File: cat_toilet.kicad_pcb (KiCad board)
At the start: 2 copper layers, 38 x 35 mm, 30 parts, among them J1 Conn_01x02, J2 ISP, J3 GP2Y0A41SK0F, Q1 S8050, SW1 EN Btn, SW2 EN Btn, SW3 Pairing Btn, U1 NCP187, U2 USB_CType_6Pin, U3 MCP73831, U4 ESP32-WROOM-32E

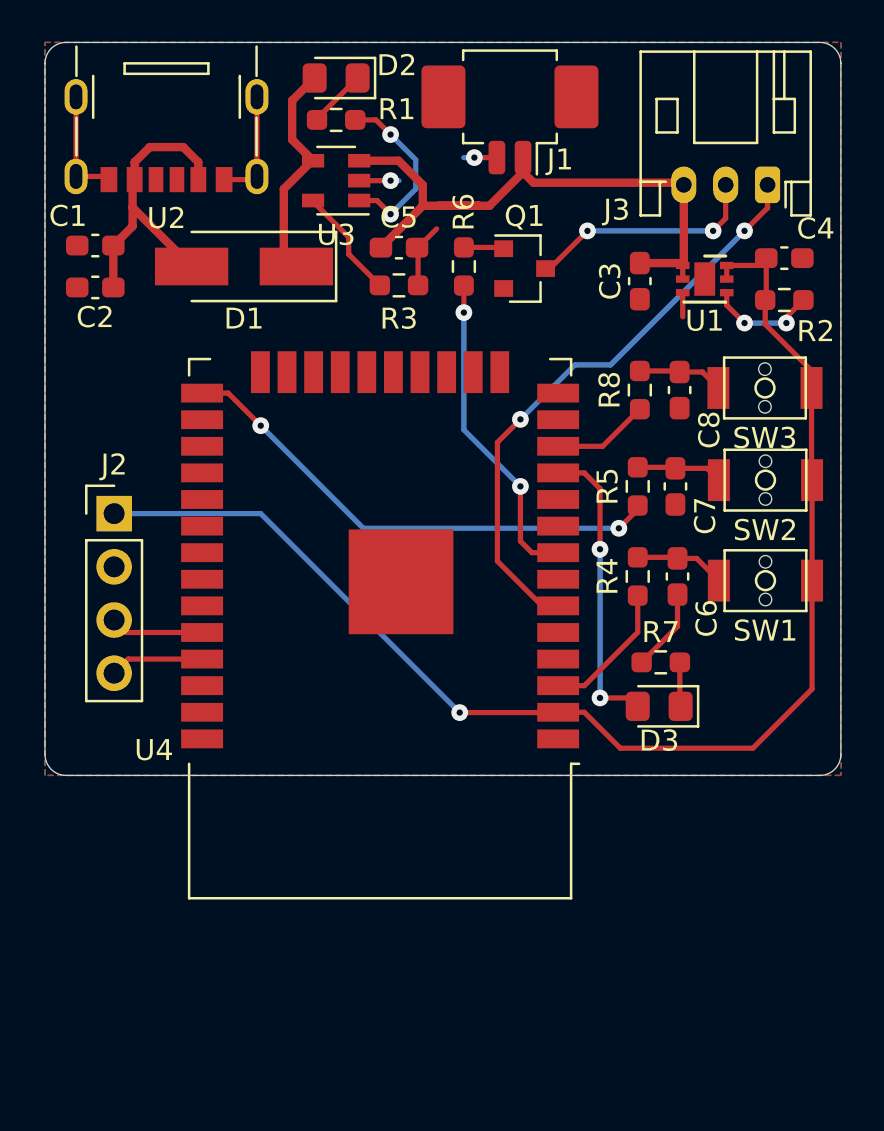
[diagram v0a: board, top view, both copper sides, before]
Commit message: 2021-12-14
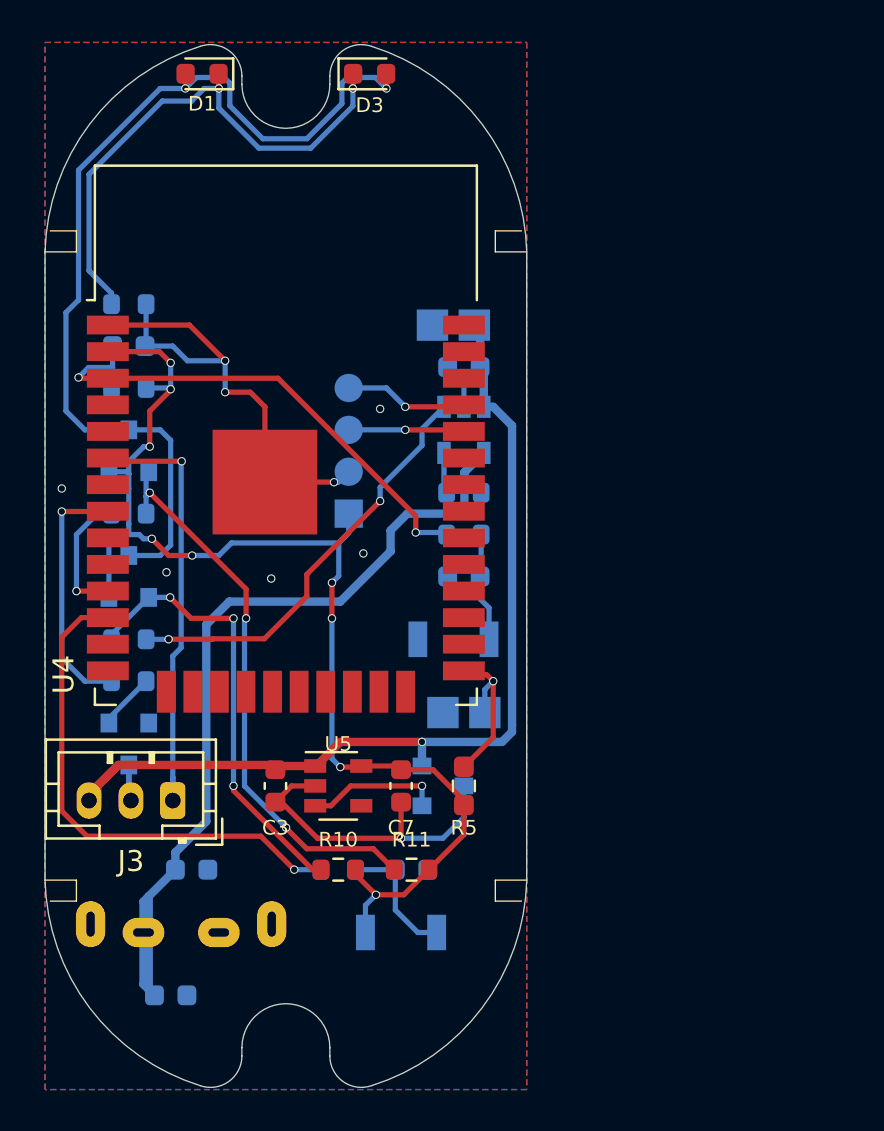
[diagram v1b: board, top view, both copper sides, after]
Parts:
- removed C4: 10u, Capacitor_SMD:C_0603_1608Metric_Pad1.08x0.95mm_HandSolder
- removed D2: LED/2012, LED_SMD:LED_0805_2012Metric_Pad1.15x1.40mm_HandSolder
- removed SW3: Pairing Btn, ali_Switch:NW3-A03-05
- added C9: 1u, Capacitor_SMD:C_0603_1608Metric, B.Cu at (4.00, 14.5)
- added Q2: BC856B,215, Package_TO_SOT_SMD:SOT-23, B.Cu at (4.00, 25.5)
- added Q3: BC856B,215, Package_TO_SOT_SMD:SOT-23, B.Cu at (4.00, 19.5)
- added R10: 33k, Resistor_SMD:R_0603_1608Metric, F.Cu at (14.0, 39.5)
- added R11: 33k, Resistor_SMD:R_0603_1608Metric, F.Cu at (17.5, 39.5)
- added R9: 33k, Resistor_SMD:R_0603_1608Metric, B.Cu at (4.00, 22.5)
- added TP1: TestPoint_2Pole, tp:boot, B.Cu at (19.0, 32.0)
- added U5: MCP1802T-3302I/OT, Package_TO_SOT_SMD:SOT-23-5, F.Cu at (14.0, 35.5)
- C1, C2, C5, C6, C8: footprint Capacitor_SMD:C_0603_1608Metric_Pad1.08x0.95mm_HandSolder -> Capacitor_SMD:C_0603_1608Metric; moved to B.Cu
- C3, C7: footprint Capacitor_SMD:C_0603_1608Metric_Pad1.08x0.95mm_HandSolder -> Capacitor_SMD:C_0603_1608Metric
- D1: value SK24/SMA -> LED/1608; footprint Diode_SMD:D_SMA_Handsoldering -> LED_SMD:LED_0603_1608Metric
- D3: value LED -> LED/1608; footprint LED_SMD:LED_0805_2012Metric_Pad1.15x1.40mm_HandSolder -> LED_SMD:LED_0603_1608Metric
- J1: value Conn_01x02 -> Batt; footprint Connector_Molex:Molex_PicoBlade_53261-0271_1x02-1MP_P1.25mm_Horizontal -> tp:boot; moved to B.Cu
- J2: footprint Connector_PinHeader_2.54mm:PinHeader_1x04_P2.54mm_Vertical -> Connector_PinHeader_2.00mm:PinHeader_1x04_P2.00mm_Vertical; moved to B.Cu
- J3: footprint Connector_JST:JST_PH_S3B-PH-K_1x03_P2.00mm_Horizontal -> Connector_JST:JST_PH_B3B-PH-K_1x03_P2.00mm_Vertical
- Q1: value S8050 -> npn; moved to B.Cu
- R1: value 510 -> 10k; footprint Resistor_SMD:R_0603_1608Metric_Pad0.98x0.95mm_HandSolder -> Resistor_SMD:R_0603_1608Metric; moved to B.Cu
- R2: value 100k -> 33k; footprint Resistor_SMD:R_0603_1608Metric_Pad0.98x0.95mm_HandSolder -> Resistor_SMD:R_0603_1608Metric; moved to B.Cu
- R3, R6, R7, R8: footprint Resistor_SMD:R_0603_1608Metric_Pad0.98x0.95mm_HandSolder -> Resistor_SMD:R_0603_1608Metric; moved to B.Cu
- R4: value 1k -> 0; footprint Resistor_SMD:R_0603_1608Metric_Pad0.98x0.95mm_HandSolder -> Resistor_SMD:R_0603_1608Metric; moved to B.Cu
- R5: value 1k -> 10k
- SW1: footprint ali_Switch:NW3-A03-05 -> Button_Switch_SMD:SW_SPST_B3U-1000P; moved to B.Cu
- SW2: value EN Btn -> Pairing Btn; footprint ali_Switch:NW3-A03-05 -> Button_Switch_SMD:SW_SPST_B3U-1000P; moved to B.Cu
- U1: value NCP187 -> MCP100-315D; footprint Package_DFN_QFN:DFN-6-1EP_2x2mm_P0.65mm_EP1x1.6mm -> Package_TO_SOT_SMD:SOT-23; moved to B.Cu
- U2: value USB_CType_6Pin -> USB_CType_2Pin; footprint ali_Connector:USB_CType_6Pin -> ali_Connector:USB_CType_2Pin; moved to B.Cu
- U3: moved to B.Cu
- moved U2 42.5 mm to (6.50, 42.5)
- moved J3 40.9 mm to (6.10, 36.2)
- moved C1 36.0 mm to (6.00, 45.5), turned to 0 degrees
- moved R2 35.2 mm to (4.00, 28.5), turned to 180 degrees
- moved D3 33.2 mm to (15.5, 1.50), turned to 0 degrees
- moved R7 30.6 mm to (4.00, 12.5), turned to 180 degrees
- moved C3 29.7 mm to (11.0, 35.5)
- moved Q1 29.5 mm to (4.00, 33.5), turned to 270 degrees
- moved C2 28.2 mm to (7.00, 39.5), turned to 0 degrees
- moved SW2 27.7 mm to (17.0, 42.5)
- moved U1 27.2 mm to (19.0, 35.5)
- moved R8 27.1 mm to (14.0, 39.5), turned to 0 degrees
- moved C8 26.2 mm to (17.5, 39.5), turned to 0 degrees
- moved R6 25.5 mm to (4.00, 30.5), turned to 180 degrees
- moved C7 19.4 mm to (17.0, 35.5)
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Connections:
- C7 pad 1: Net-(C7-Pad1) -> +3V3
- D1 pad 2: VBUS -> Net-(D1-Pad2)
- D3 pad 1: Net-(D3-Pad1) -> Net-(D1-Pad1)
- D3 pad 2: LED -> Net-(D1-Pad2)
- R1 pad 1: Net-(D2-Pad1) -> EN
- R1 pad 2: Net-(R1-Pad2) -> +3V3
- R2 pad 1: +3V3 -> CHRG
- R2 pad 2: Net-(R2-Pad2) -> Net-(Q2-Pad1)
- R5 pad 2: Net-(C7-Pad1) -> +3V3
- R7 pad 2: Net-(D3-Pad1) -> Net-(D1-Pad1)
- SW1 pad 1: +3V3 -> Earth
- SW2 pad 2: Net-(C7-Pad1) -> Net-(C8-Pad1)
- U1 pad 1: BATT -> Net-(U1-Pad1)
- U3 pad 1: Net-(R1-Pad2) -> CHRG
- U3 pad 4: Net-(D1-Pad1) -> VBUS
- U4 pad 10: Net-(U4-Pad10) -> (no net)
- U4 pad 13: Net-(U4-Pad13) -> (no net)
- U4 pad 14: Net-(U4-Pad14) -> (no net)
- U4 pad 16: Net-(U4-Pad16) -> (no net)
- U4 pad 17: Net-(U4-Pad17) -> (no net)
- U4 pad 18: Net-(U4-Pad18) -> (no net)
- U4 pad 19: Net-(U4-Pad19) -> (no net)
- U4 pad 20: Net-(U4-Pad20) -> (no net)
- U4 pad 21: Net-(U4-Pad21) -> (no net)
- U4 pad 22: Net-(U4-Pad22) -> (no net)
- U4 pad 23: Net-(U4-Pad23) -> (no net)
- U4 pad 24: Net-(U4-Pad24) -> (no net)
- U4 pad 26: Net-(U4-Pad26) -> (no net)
- U4 pad 27: Net-(U4-Pad27) -> (no net)
- U4 pad 28: Net-(U4-Pad28) -> (no net)
- U4 pad 29: Net-(U4-Pad29) -> (no net)
- U4 pad 30: Net-(U4-Pad30) -> (no net)
- U4 pad 31: Net-(U4-Pad31) -> (no net)
- U4 pad 32: Net-(U4-Pad32) -> (no net)
- U4 pad 33: Net-(U4-Pad33) -> (no net)
- U4 pad 36: Net-(U4-Pad36) -> (no net)
- U4 pad 37: Net-(U4-Pad37) -> (no net)
- U4 pad 4: Net-(U4-Pad4) -> (no net)
- U4 pad 5: Net-(U4-Pad5) -> (no net)
- U4 pad 7: Net-(U4-Pad7) -> (no net)
- U4 pad 9: Net-(U4-Pad9) -> (no net)
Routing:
- net Net-(D1-Pad2): track 0.00 -> 46.3 mm, vias 0 -> 2
- net VBUS: track 15.0 -> 42.1 mm
- net Net-(Q3-Pad1): track 0.00 -> 27.1 mm, vias 0 -> 3
- net Net-(Q2-Pad1): track 0.00 -> 21.2 mm, vias 0 -> 3
- net CHRG: track 0.00 -> 20.3 mm, vias 0 -> 2
- net BTN: track 4.63 -> 24.4 mm, vias 0 -> 1
- net Earth: track 22.6 -> 41.7 mm, vias 2 -> 9
- net EN: track 6.61 -> 25.0 mm, vias 0 -> 2
- net BOOT: track 24.0 -> 7.94 mm, vias 2 -> 1
- net BATT: track 30.2 -> 45.4 mm, vias 0 -> 1
- net Net-(D1-Pad1): track 11.1 -> 25.8 mm, vias 0 -> 2
- net Net-(R1-Pad2): track 8.54 -> 0.00 mm, vias 2 -> 0
- net Net-(J3-Pad2): track 11.3 -> 3.28 mm, vias 2 -> 0
- net LED: track 14.3 -> 6.29 mm, vias 2 -> 1
- net IR_SENS: track 28.2 -> 20.9 mm, vias 2 -> 1
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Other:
- board size 38 x 35 mm -> 23 x 49.8 mm
- net class Default: via_dia 0.8 -> 0.4
- net class pwr: clearance 0.3 -> 0.2; via_dia 0.8 -> 0.4; via_drill 0.4 -> 0.3
- board text added: "+"
- board text added: "-"
- board text added: "g"
- board text added: "r"
- board text added: "t"
- board text added: "v"
